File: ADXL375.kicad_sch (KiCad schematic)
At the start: 1 part, among them U6 ADXL372BCCZ-RL

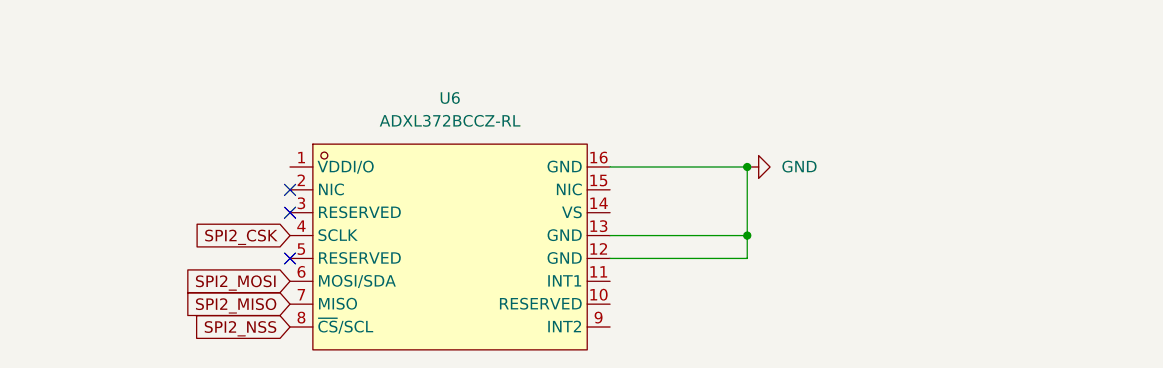
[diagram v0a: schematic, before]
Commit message: INA SENSOR
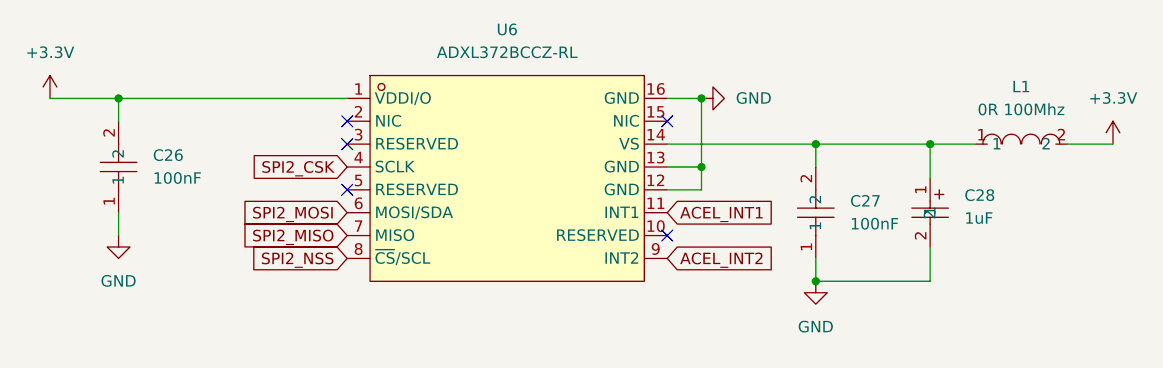
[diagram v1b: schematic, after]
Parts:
- added C26, C27: 100nF, easyeda2kicad:C0402, symbol CANSAT_STM32_symbols:TCC0402X7R104J500AT
- added C28: 1uF, easyeda2kicad:CAP-SMD_L3.5-W2.8-R-RD, symbol CANSAT_STM32_symbols:TAJB105K035RNJ
- added L1: 0R 100Mhz, easyeda2kicad:L0402, symbol CANSAT_STM32_symbols:CBG100505U000T
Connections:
- net GND: now also C26.1, C27.1, C28.2
- net +3.3V: now reaches U6.1 (VDDI/O)
- net +3.3V: now also C26.2, L1.2
- net ACEL_INT1: now reaches U6.11 (INT1)
- net at U6.14 (VS): now also C27.2, C28.1, L1.1
- net ACEL_INT2: now reaches U6.9 (INT2)
- no-connect marks 3 -> 5
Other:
- moved on the sheet: U6
